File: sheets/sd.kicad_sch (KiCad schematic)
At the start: 1 part

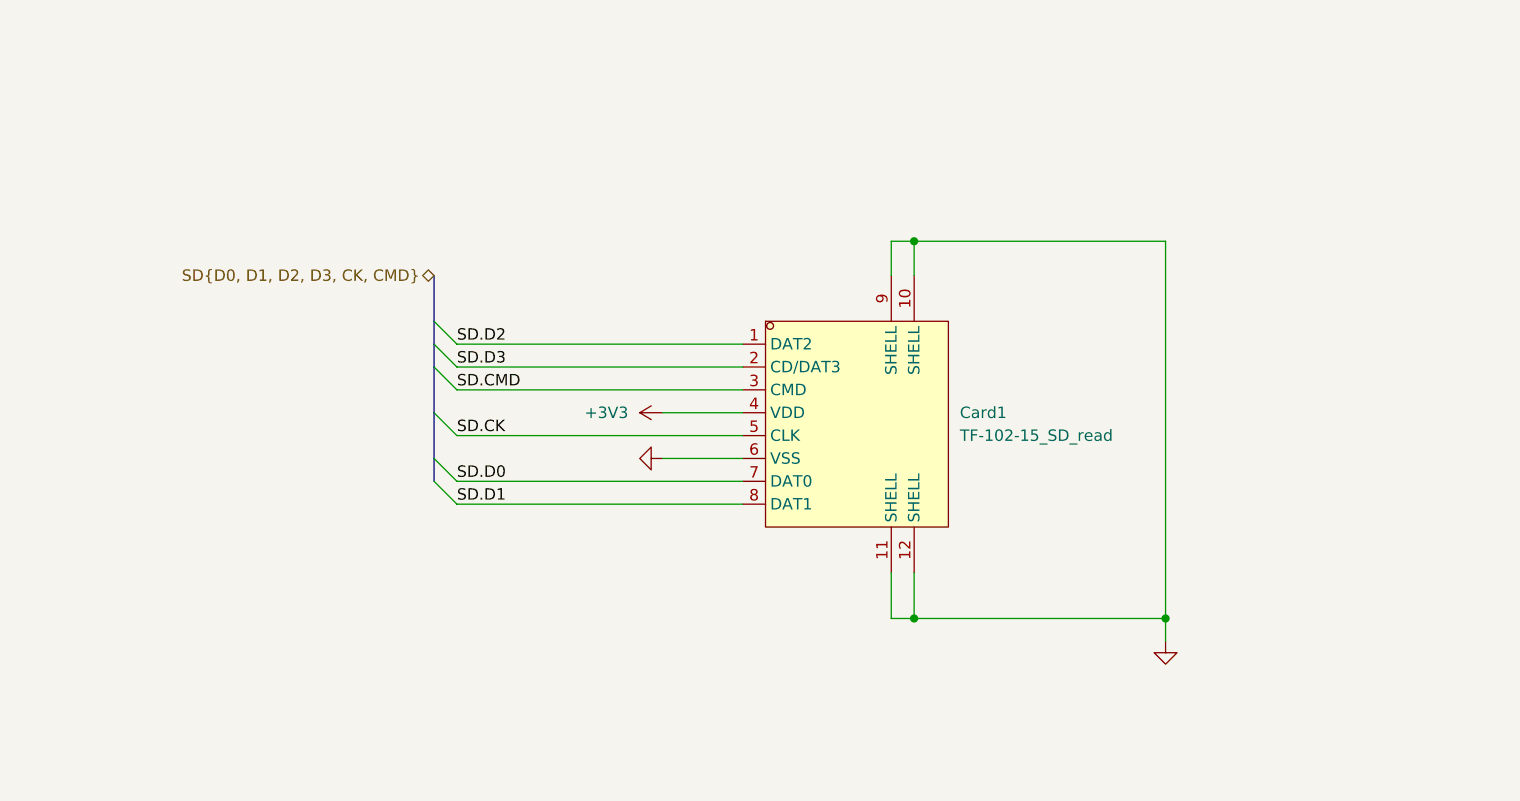
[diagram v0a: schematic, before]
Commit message: added spi
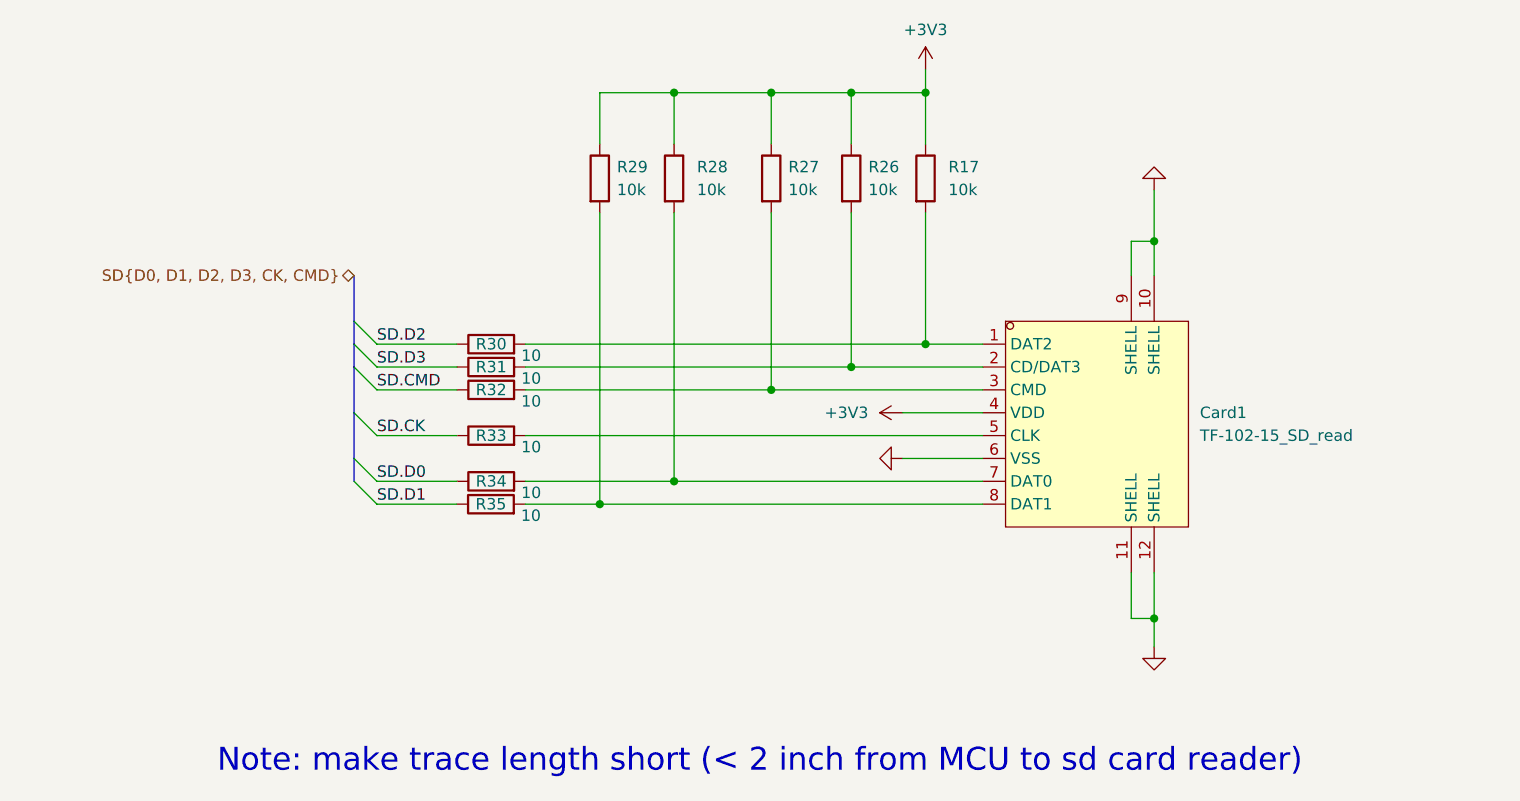
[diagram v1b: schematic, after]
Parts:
- added R17, R26, R27, R28, R29: 10k, symbol Device:R
- added R30, R31, R32, R33, R34, R35: 10, symbol Device:R
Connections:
- net +3V3: now also R17.1, R26.1, R27.1, R28.1, R29.1
- net SD.CK: now also R33.1; no longer Card1.5 (CLK)
- net SD.CMD: now also R32.1; no longer Card1.3 (CMD)
- net SD.D0: now also R34.1; no longer Card1.7 (DAT0)
- net SD.D1: now also R35.1; no longer Card1.8 (DAT1)
- net SD.D2: now also R30.1; no longer Card1.1 (DAT2)
- net SD.D3: now also R31.1; no longer Card1.2 (CD/DAT3)
- new net: Card1.7 (DAT0), R28.2, R34.2
- new net: Card1.2 (CD/DAT3), R26.2, R31.2
- new net: Card1.8 (DAT1), R29.2, R35.2
- new net: Card1.3 (CMD), R27.2, R32.2
- new net: Card1.1 (DAT2), R17.2, R30.2
- new net: Card1.5 (CLK), R33.2
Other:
- note added: "Note: make trace length short (< 2 inch from MCU to sd card reader)"
- moved on the sheet: Card1

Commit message: Rev1 schematic done
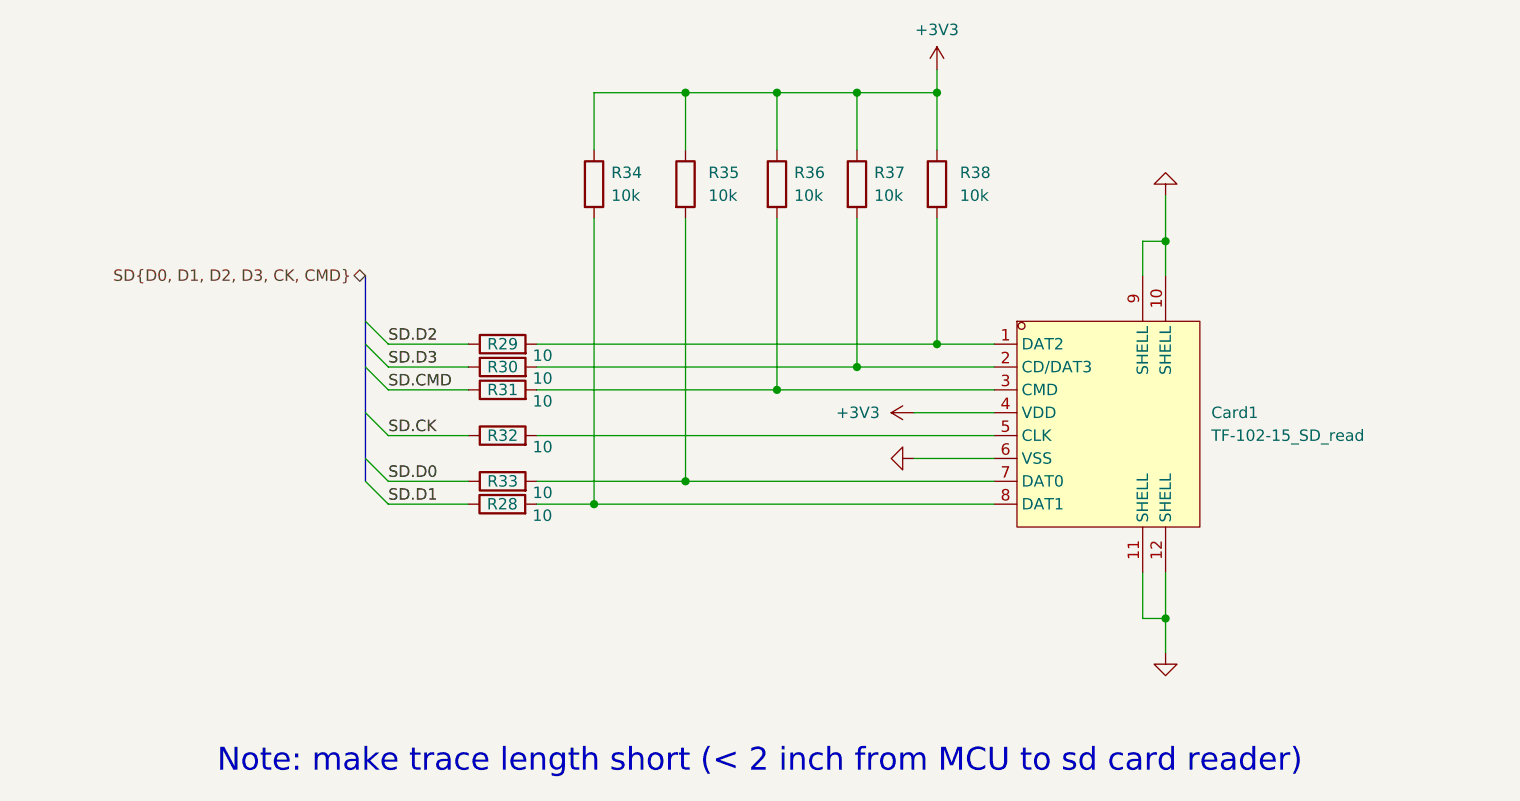
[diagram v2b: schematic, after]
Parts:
- renumbered R35 to R28, R30 to R29, R31 to R30, R32 to R31, R33 to R32, R34 to R33, R29 to R34, R28 to R35, R27 to R36, R26 to R37, R17 to R38
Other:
- moved on the sheet: Card1, R28, R29, R30, R31, R32, R33, R34, R35, R36, R37, R38
